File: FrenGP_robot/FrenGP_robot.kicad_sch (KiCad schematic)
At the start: 19 parts, among them J1 Screw_Terminal_01x02, J2 Screw_Terminal_01x02, J3 Screw_Terminal_01x02, SW1 SW_Push

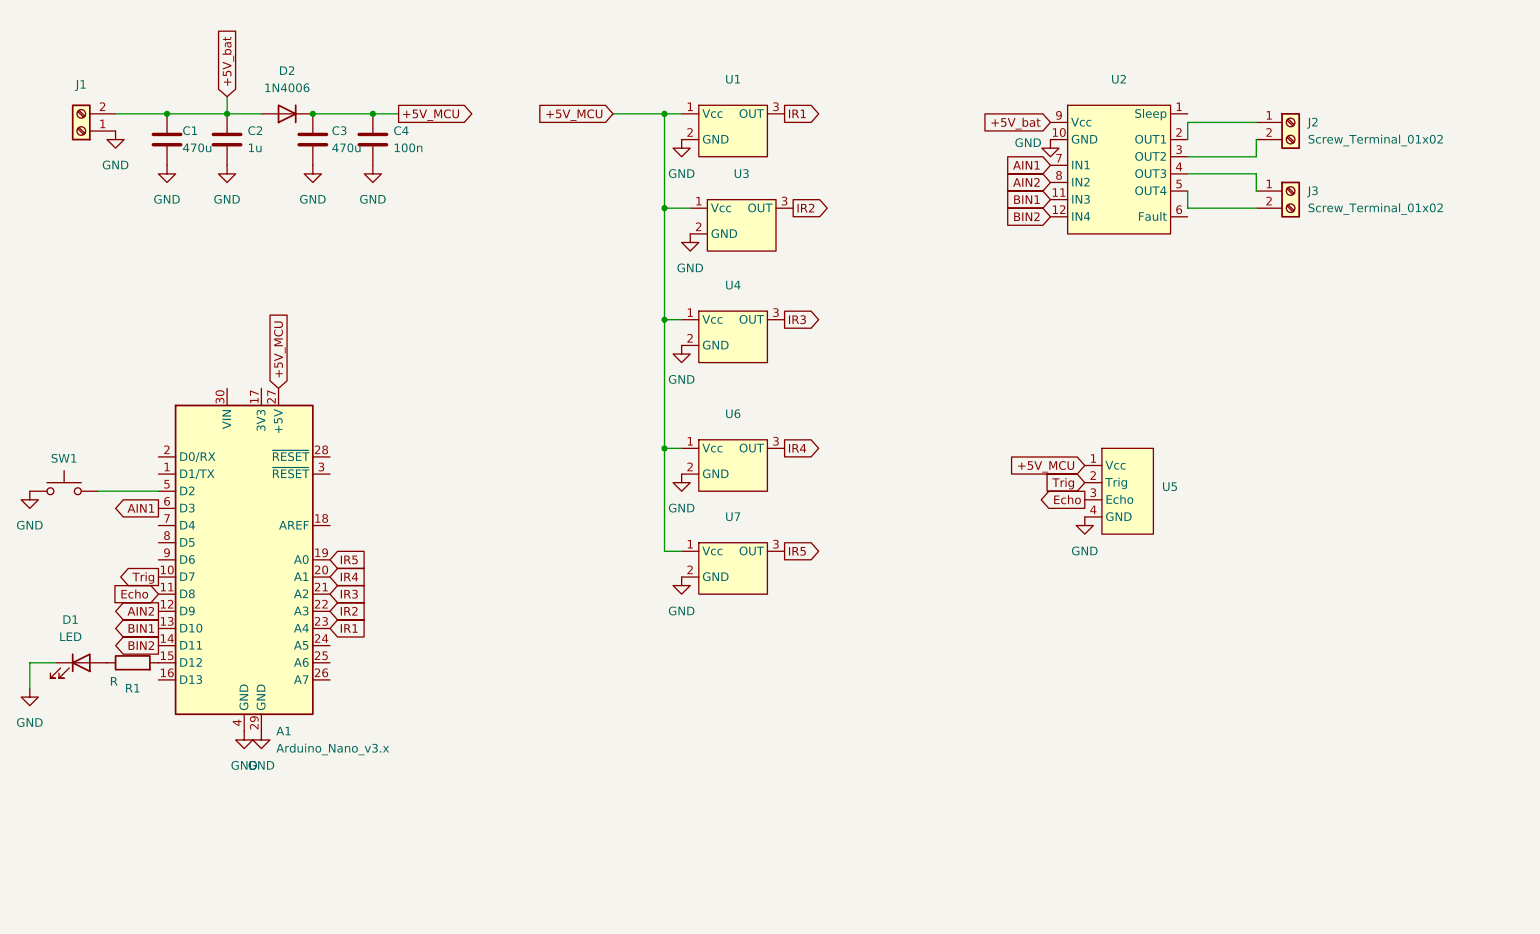
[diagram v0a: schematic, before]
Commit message: Update v1.1
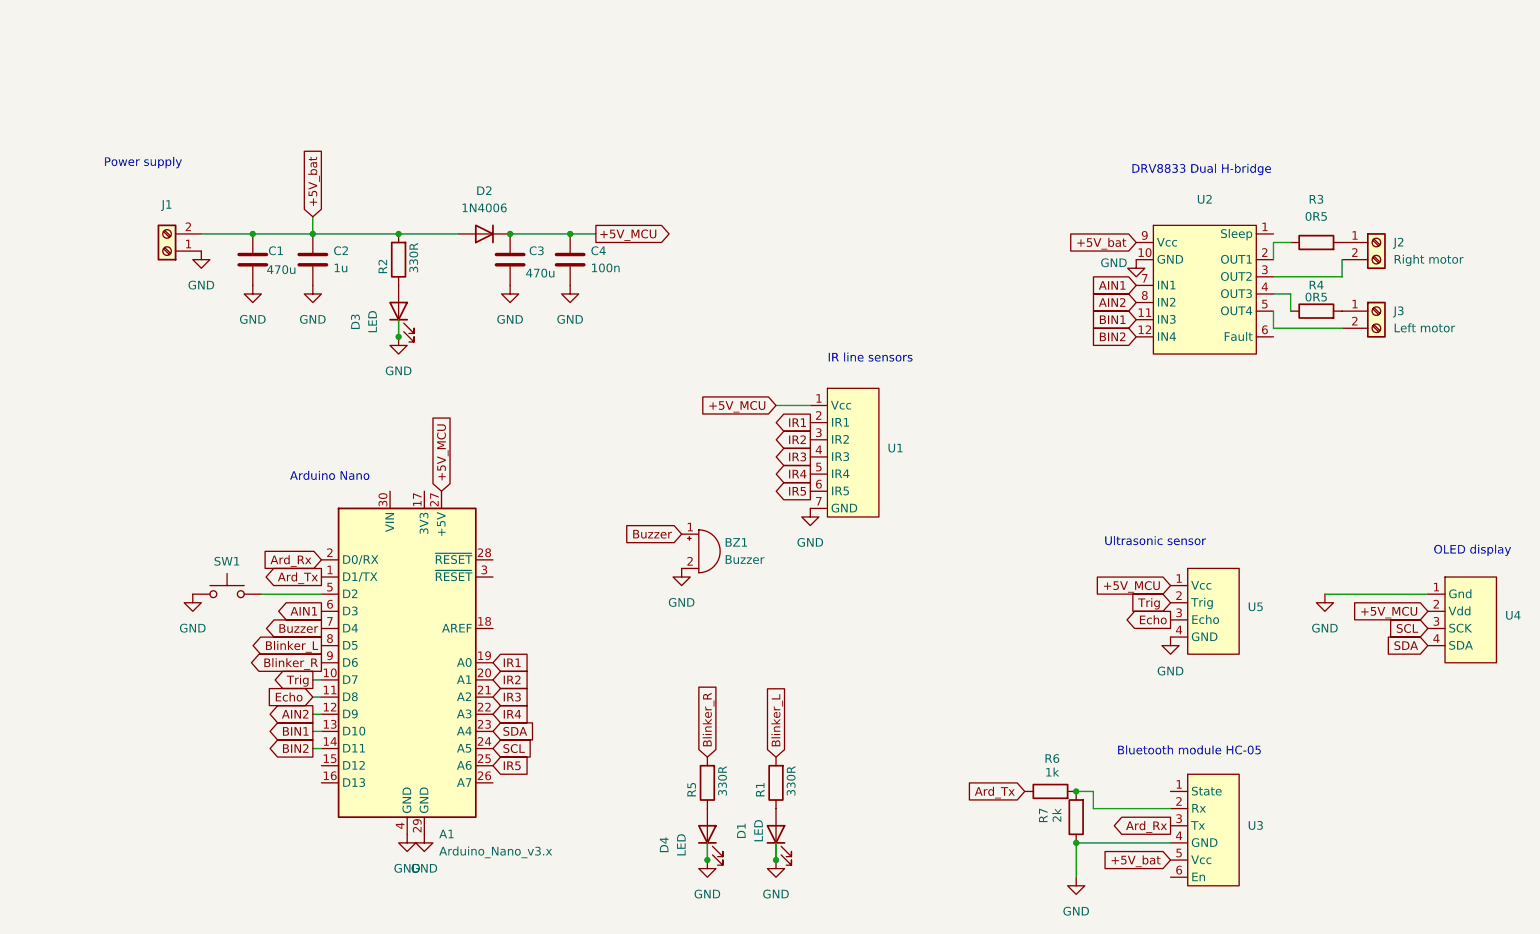
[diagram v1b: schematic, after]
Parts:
- removed U1, U3, U4, U6, U7: ~, DRV_8833_module:3pin_Reflection_sensor, symbol DRV_8833:3pin_reflection_sensor
- added BZ1: Buzzer, Buzzer_Beeper:Buzzer_12x9.5RM7.6, symbol Device:Buzzer
- added D3, D4: LED, Diode_SMD:D_0603_1608Metric_Pad1.05x0.95mm_HandSolder, symbol Device:LED
- added R2, R5: 330R, Resistor_SMD:R_0603_1608Metric_Pad0.98x0.95mm_HandSolder, symbol Device:R
- added R3, R4: 0R5, Resistor_SMD:R_0805_2012Metric_Pad1.20x1.40mm_HandSolder, symbol Device:R
- added R6: 1k, Resistor_SMD:R_0603_1608Metric_Pad0.98x0.95mm_HandSolder, symbol Device:R
- added R7: 2k, Resistor_SMD:R_0603_1608Metric_Pad0.98x0.95mm_HandSolder, symbol Device:R
- added U1: ~, DRV_8833_module:IR sensor header, symbol DRV_8833:5Ch_IR_sensor
- added U3: ~, DRV_8833_module:HC-05 header, symbol DRV_8833:HC-05
- added U4: ~, DRV_8833_module:OLED display header, symbol DRV_8833:OLED_header
- J2: value Screw_Terminal_01x02 -> Right motor
- J3: value Screw_Terminal_01x02 -> Left motor
- R1: value R -> 330R
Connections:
- net +5V_MCU: now also U1.1 (Vcc), U4.2 (Vdd)
- net +5V_bat: now also R2.2, U3.5 (Vcc)
- net GND: now also BZ1.2 (-), D3.1 (K), D4.1 (K), R7.1, U1.7 (GND), U3.4 (GND), U4.1 (Gnd)
- net IR1: now also A1.19 (A0), U1.2 (IR1); no longer A1.23 (A4)
- net IR2: now also A1.20 (A1), U1.3 (IR2); no longer A1.22 (A3)
- net IR3: now also U1.4 (IR3)
- net IR4: now also A1.22 (A3), U1.5 (IR4); no longer A1.20 (A1)
- net IR5: now also A1.25 (A6), U1.6 (IR5); no longer A1.19 (A0)
- net at J3.1 (Pin_1): now also R4.2; no longer U2.4 (OUT3)
- net at J2.1 (Pin_1): now also R3.2; no longer U2.2 (OUT1)
- net Ard_Tx: now reaches A1.1 (D1/TX)
- net Ard_Tx: now also R6.1
- net at A1.15 (D12): no longer R1.2
- net Ard_Rx: now reaches A1.2 (D0/RX)
- net Ard_Rx: now also U3.3 (Tx)
- net SCL: now reaches A1.24 (A5)
- net SCL: now also U4.3 (SCK)
- net Buzzer: now reaches A1.7 (D4)
- net Buzzer: now also BZ1.1 (+)
- net Blinker_L: now reaches A1.8 (D5)
- net Blinker_L: now also R1.2
- net Blinker_R: now reaches A1.9 (D6)
- net Blinker_R: now also R5.2
- new net: R4.1, U2.4 (OUT3)
- new net: R6.2, R7.2, U3.2 (Rx)
- new net: R3.1, U2.2 (OUT1)
- new net: D4.2 (A), R5.1
- new net: D3.2 (A), R2.1
- new net SDA: A1.23 (A4), U4.4 (SDA)
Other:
- note added: "Arduino Nano"
- note added: "Bluetooth module HC-05"
- note added: "DRV8833 Dual H-bridge"
- note added: "IR line sensors"
- note added: "OLED display"
- note added: "Power supply"
- note added: "Ultrasonic sensor"
- moved on the sheet: A1, C1, C2, C3, C4, D1, D2, J1, J2, J3, R1, SW1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
